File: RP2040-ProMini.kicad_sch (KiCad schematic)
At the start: 40 parts, among them J1 CONN_L, J2 CONN_U, J3 CONN_R2, J4 CONN_R, Q1 AO3400A, U1 W25Q128JVS, U2 RP2040, U3 TPS63060, U4 W25Q128JVEIQ, Y1 12MHz

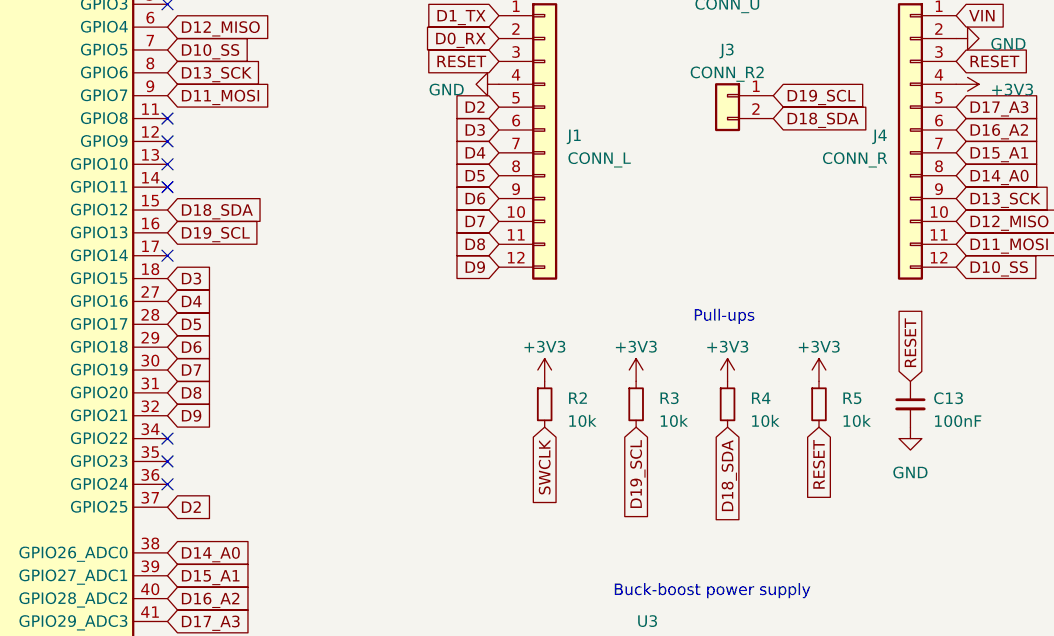
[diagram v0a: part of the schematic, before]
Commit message: Added D20 and D21. Fixed minor issues. Moved stuff around.
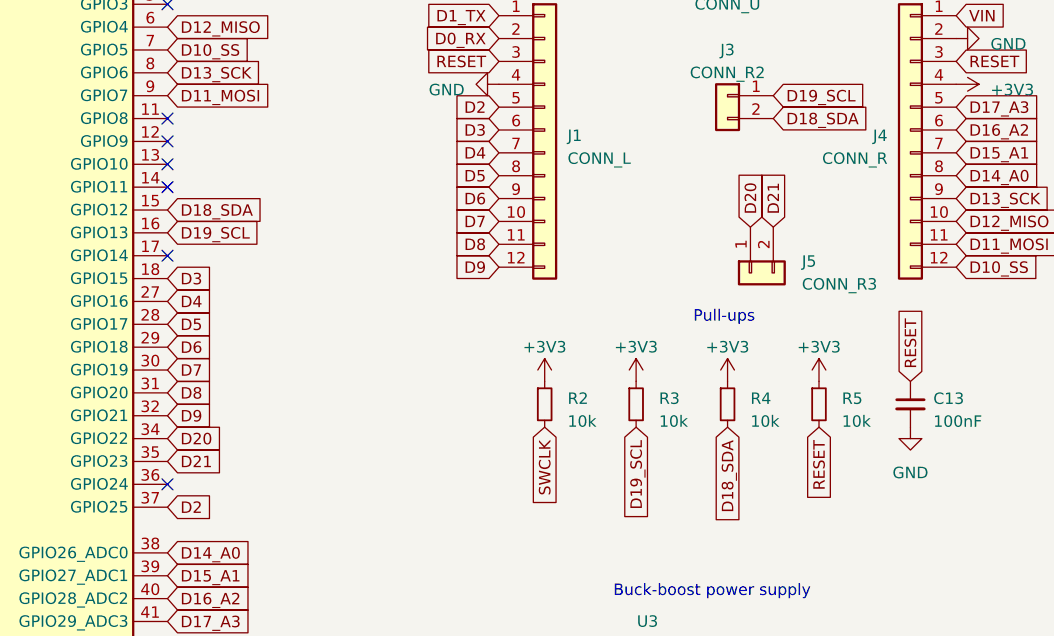
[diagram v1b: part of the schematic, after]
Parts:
- added J5: CONN_R3, Connector_PinHeader_2.54mm:PinHeader_1x02_P2.54mm_Vertical, symbol Connector_Generic:Conn_01x02
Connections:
- net D20: now reaches U2.34 (GPIO22)
- net D20: now also J5.1 (Pin_1)
- net D21: now reaches U2.35 (GPIO23)
- net D21: now also J5.2 (Pin_2)
- no-connect marks 10 -> 8
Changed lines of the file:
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@@
   (junction (at 151.13 39.37) (diameter 0) (color 0 0 0 0)
   )
-  (no_connect (at 166.37 102.87))
   (no_connect (at 166.37 54.61))
   (no_connect (at 166.37 52.07))
@@
   (no_connect (at 166.37 67.31))
   (no_connect (at 166.37 107.95))
-  (no_connect (at 166.37 105.41))
   (wire (pts (xy 233.68 130.81) (xy 242.57 130.81))
     (stroke (width 0) (type default))
@@
     )
   )
+  (global_label "D20" (shape input) (at 231.14 79.375 90) (fields_autoplaced)
+    (effects (font (size 1.27 1.27)) (justify left))
+    (property "Intersheetrefs" "${INTERSHEET_REFS}" (at 231.14 72.7802 90)
+      (effects (font (size 1.27 1.27)) (justify left) hide)
+    )
+  )
   (global_label "QSPI_SD3" (shape input) (at 31.75 99.06 180) (fields_autoplaced)
     (effects (font (size 1.27 1.27)) (justify right))
@@
     )
   )
+  (global_label "D20" (shape input) (at 166.37 102.87 0) (fields_autoplaced)
+    (effects (font (size 1.27 1.27)) (justify left))
+    (property "Intersheetrefs" "${INTERSHEET_REFS}" (at 172.9648 102.87 0)
+      (effects (font (size 1.27 1.27)) (justify left) hide)
+    )
+  )
   (global_label "VIN" (shape input) (at 254 55.88 0) (fields_autoplaced)
     (effects (font (size 1.27 1.27)) (justify left))
@@
     )
   )
+  (global_label "D21" (shape input) (at 166.37 105.41 0) (fields_autoplaced)
+    (effects (font (size 1.27 1.27)) (justify left))
+    (property "Intersheetrefs" "${INTERSHEET_REFS}" (at 172.9648 105.41 0)
+      (effects (font (size 1.27 1.27)) (justify left) hide)
+    )
+  )
   (global_label "D0_RX" (shape input) (at 203.2 58.42 180) (fields_autoplaced)
     (effects (font (size 1.27 1.27)) (justify right))
@@
     (effects (font (size 1.27 1.27)) (justify left))
     (property "Intersheetrefs" "${INTERSHEET_REFS}" (at 171.7553 97.79 0)
+      (effects (font (size 1.27 1.27)) (justify left) hide)
+    )
+  )
+  (global_label "D21" (shape input) (at 233.68 79.375 90) (fields_autoplaced)
+    (effects (font (size 1.27 1.27)) (justify left))
+    (property "Intersheetrefs" "${INTERSHEET_REFS}" (at 233.68 72.7802 90)
       (effects (font (size 1.27 1.27)) (justify left) hide)
     )
@@
         )
       )
+    )
+  )
+  (symbol (lib_id "Connector_Generic:Conn_01x02") (at 231.14 84.455 90) (mirror x) (unit 1)
+    (in_bom yes) (on_board yes) (dnp no)
+    (property "Reference" "J5" (at 236.855 83.185 90)
+      (effects (font (size 1.27 1.27)) (justify right))
+    )
+    (property "Value" "CONN_R3" (at 236.855 85.725 90)
+      (effects (font (size 1.27 1.27)) (justify right))
+    )
+    (property "Footprint" "Connector_PinHeader_2.54mm:PinHeader_1x02_P2.54mm_Vertical" (at 231.14 84.455 0)
+      (effects (font (size 1.27 1.27)) hide)
+    )
+    (property "Datasheet" "~" (at 231.14 84.455 0)
+      (effects (font (size 1.27 1.27)) hide)
+    )
+    (pin "1")
+    (pin "2")
+    (instances
+      (project "RP2040-ProMini"
+        (path "/9a38a81c-7302-494f-9784-2ab4342a0a1d"
+          (reference "J5") (unit 1)
+        )
+      )
